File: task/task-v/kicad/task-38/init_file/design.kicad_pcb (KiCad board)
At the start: 3 copper layers, 150 x 120 mm, 4 parts, among them U1 STM32F103, Y1 8MHz

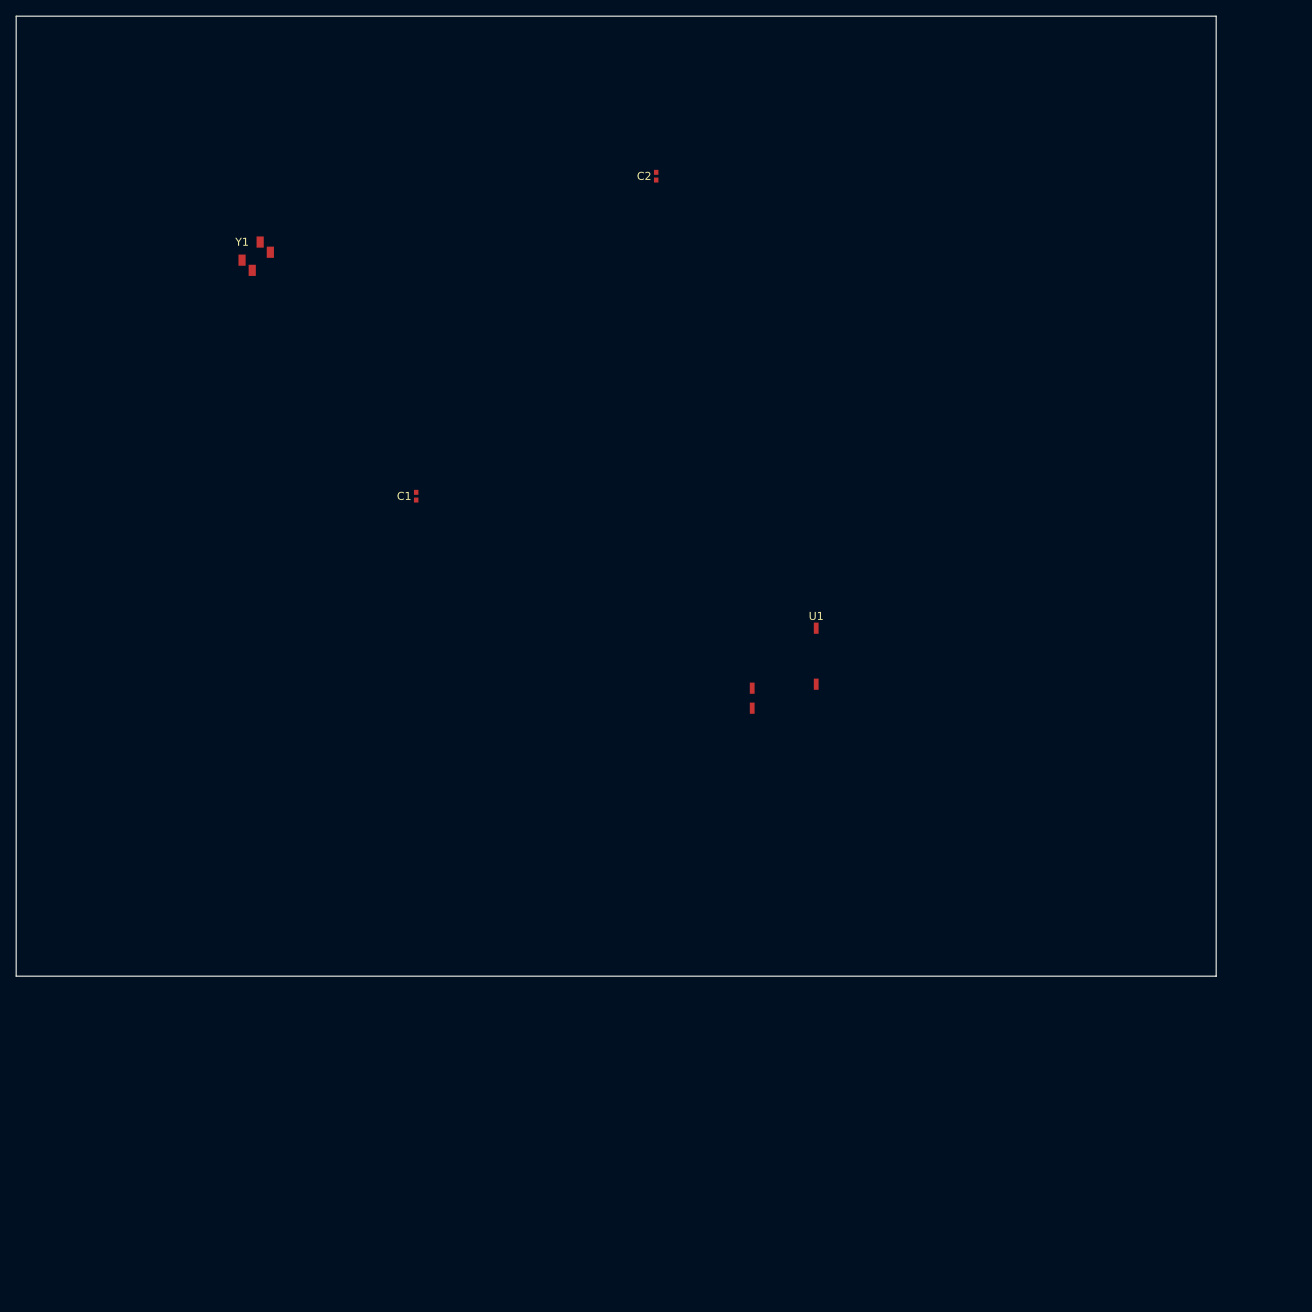
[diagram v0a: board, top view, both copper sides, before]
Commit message: Refine engineering task metadata and instructions
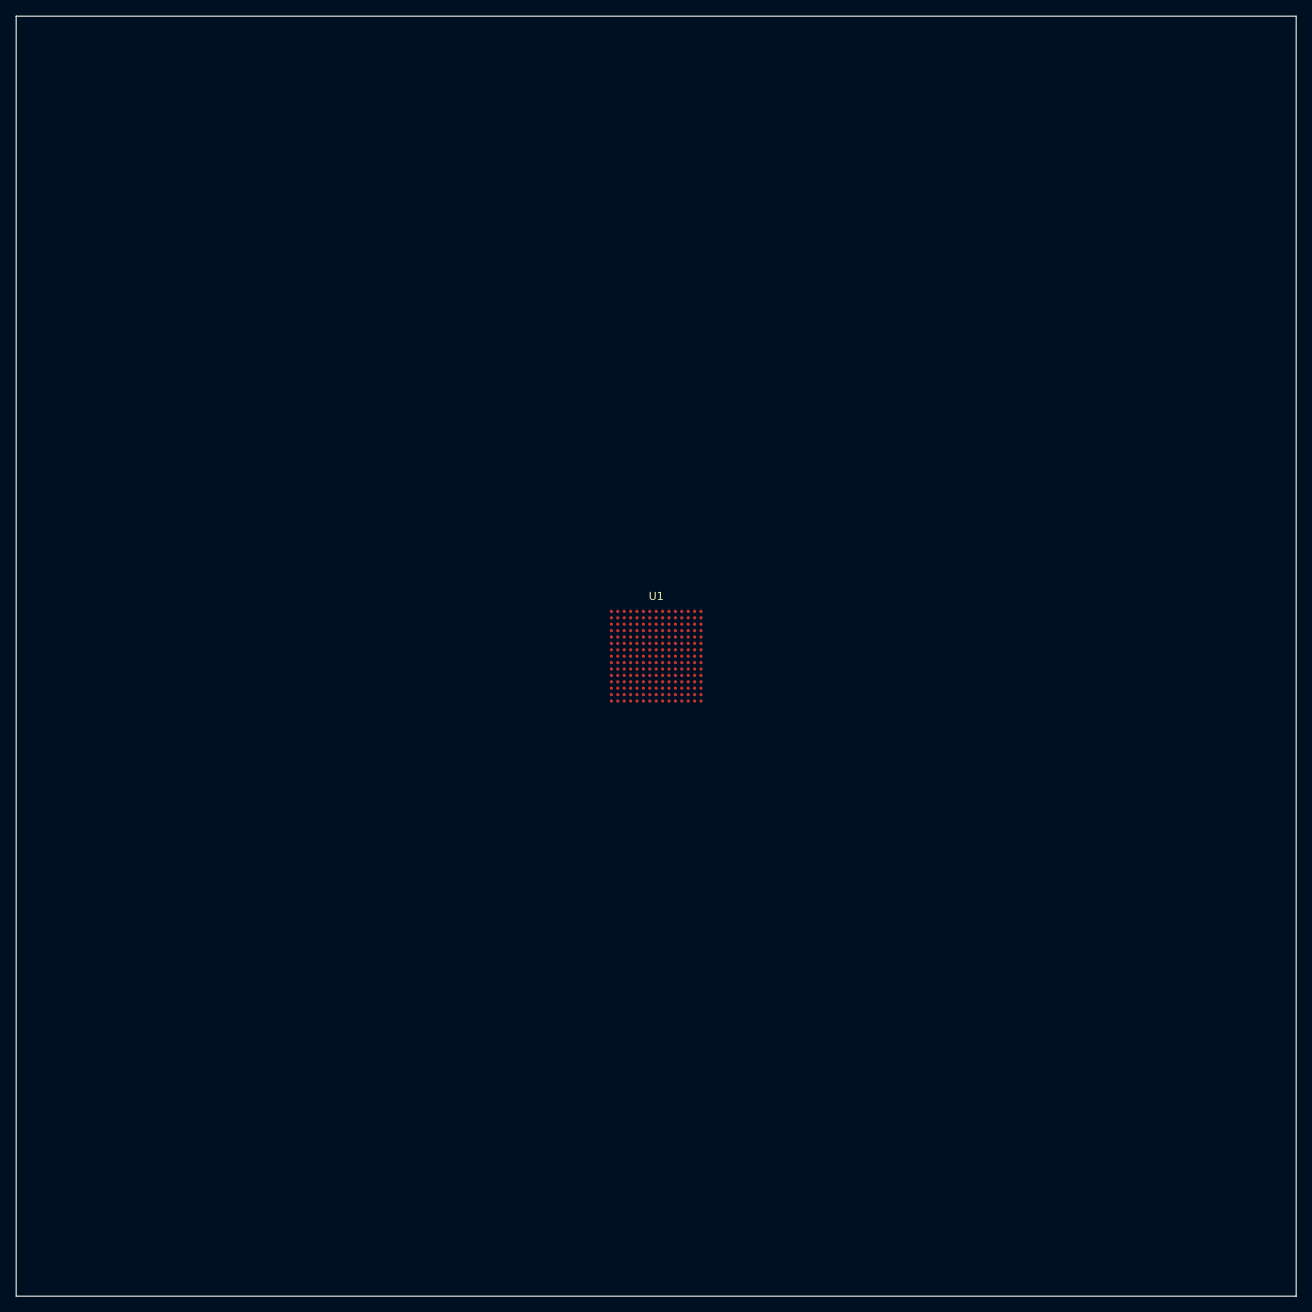
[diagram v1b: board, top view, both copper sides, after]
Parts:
- removed C1, C2: 12pF, Capacitor_SMD:C_0402_1005Metric
- removed Y1: 8MHz, Crystal:Crystal_SMD_3225-4Pin_3.2x2.5mm
- U1: value STM32F103 -> BGA-225; footprint Package_QFP:LQFP-48_7x7mm_P0.5mm -> Package_BGA:BGA-225_15x15_P0.8mm
- moved U1 20.0 mm to (80.0, 80.0)
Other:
- board size 150 x 120 mm -> 160 x 160 mm
- copper layers 3 -> 4
